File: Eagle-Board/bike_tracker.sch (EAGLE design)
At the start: 89 parts, among them IC1 24C00TS, IC2 BME280, J1 TRANSFLASH-LOCK, Q1 IRLML5203, Q2 IRLML5203, Q3 IRLML5203, Q4 IRLML5203, U1 MPU-9250

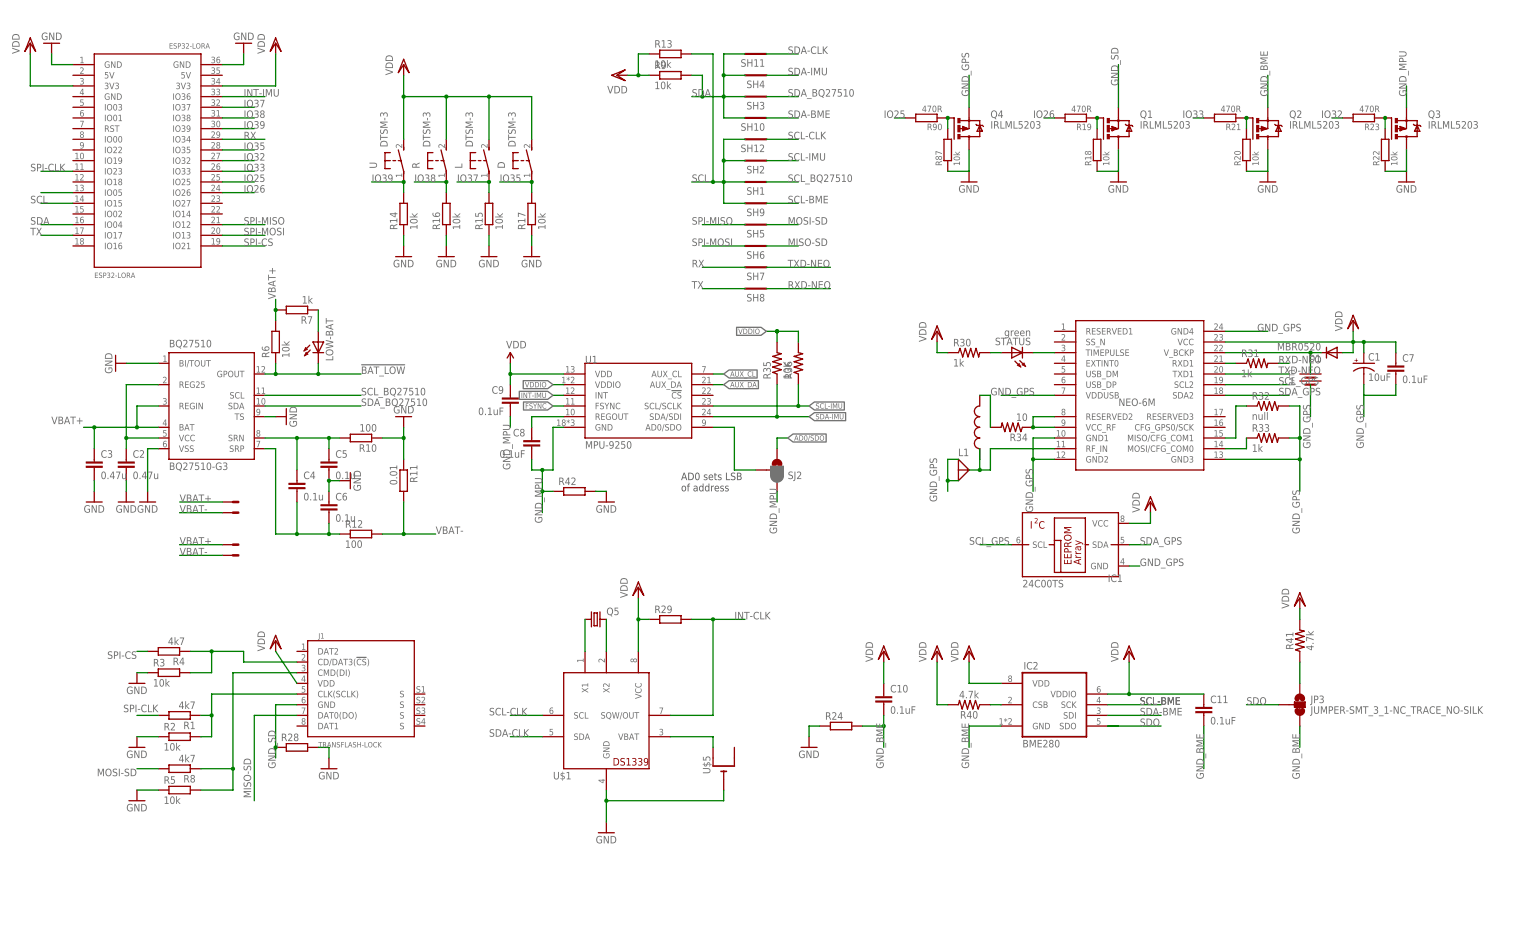
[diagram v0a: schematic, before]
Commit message: modified and cleaned for production
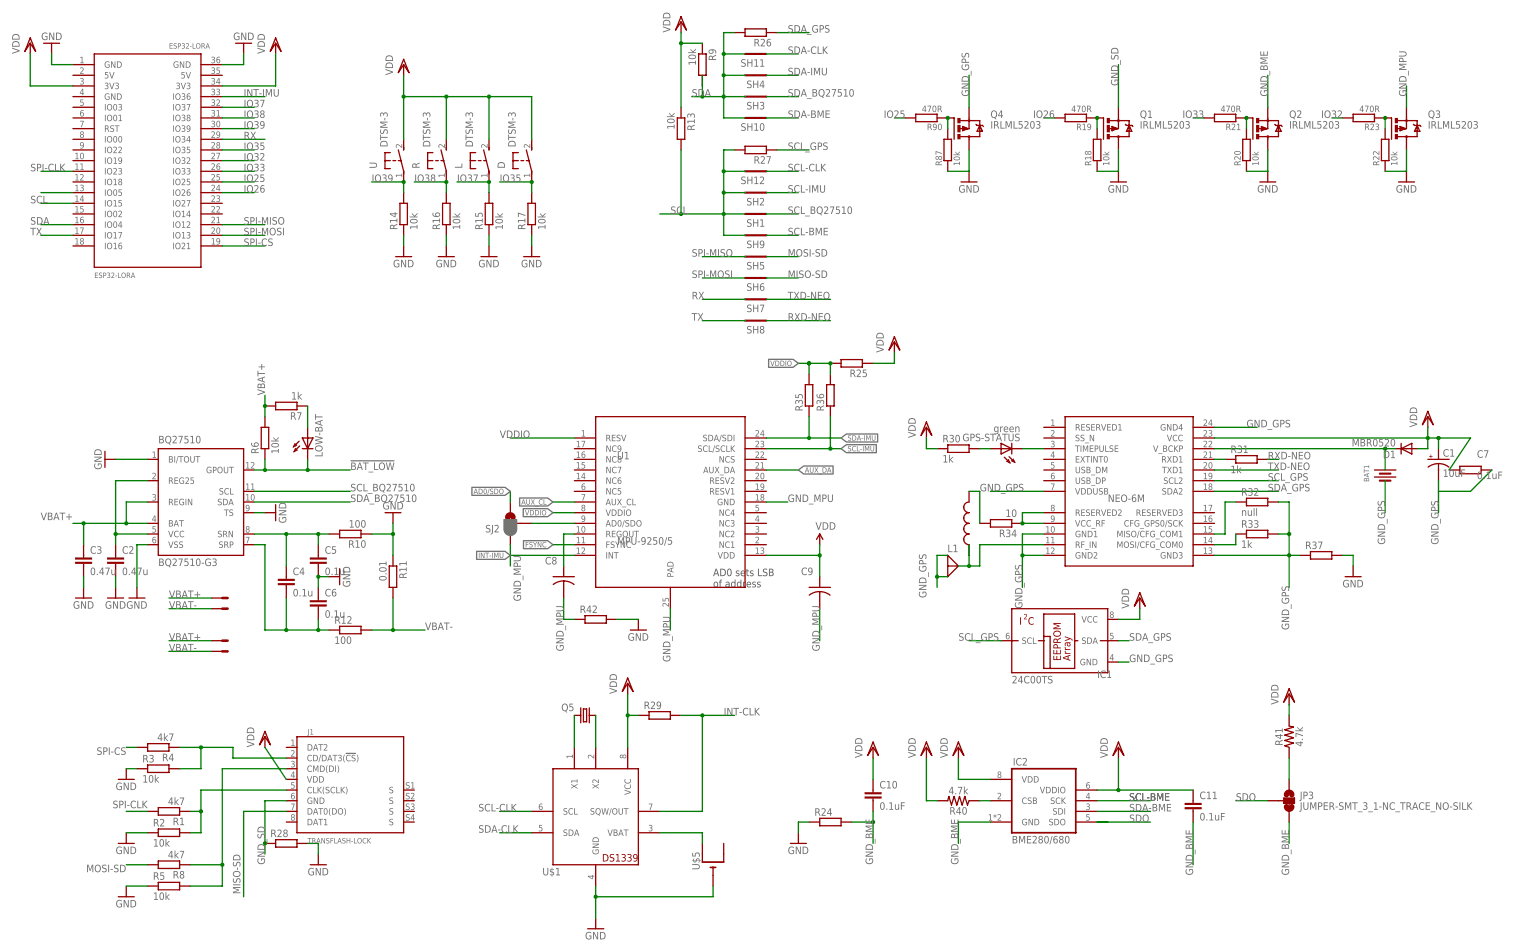
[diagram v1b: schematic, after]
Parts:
- removed STATUS: green, microduino:LED0805
- removed U$6: BLOX-NEO-6M, microduino:BLOX-NEO-6M
- added GPS-STATUS: green, microduino:LED0805
- added NEO-GPS: BLOX-NEO-6M, microduino:BLOX-NEO-6M
- added R25, R26, R27, R37: (no value), resistor:R-EU_R0201
- C7: device microduino:CAP0603-CAP -> rcl:R-EU_R0603
- C8, C9: device SparkFun-Capacitors:0.1UF-25V(+80/-20%)(0603) -> resistor:C-USC0603K
- IC2: value BME280 -> BME280/680
- R18, R19, R22, R23, R87, R90: device ssmd:R_SMDR0603 -> resistor:R-EU_R0603
- R20, R21: device ssmd:R_SMDR0603 -> rcl:R-EU_R0603
- R30: device microduino:RESISTOR0603-RES -> resistor:R-EU_R0603
- R31, R32, R33, R34: device microduino:RESISTOR0603-RES -> rcl:R-EU_R0603
- R35, R36: device SparkFun-Resistors:10KOHM-1/10W-1%(0603)0603 -> resistor:R-EU_R0603
- U1: value MPU-9250 -> MPU-9250/5; device Testing:MPU-9250 -> invensense:MPU-9250
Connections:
- net ADSD_STUB renamed N$27
- net GND: now also R37.2
- net GND_GPS: now also NEO-GPS.GND1, NEO-GPS.GND2, NEO-GPS.GND3, NEO-GPS.GND4, NEO-GPS.VDDUSB, R37.1; no longer U$6.GND1, U$6.GND2, U$6.GND3, U$6.GND4, U$6.VDDUSB
- net GND_MPU: now also U1.PAD
- net N$10: now also U$1.X2; no longer U$1.X1
- net N$13: now also U$1.X1; no longer U$1.X2
- net N$16: now also GPS-STATUS.A; no longer STATUS.A
- net N$17: now also GPS-STATUS.C, NEO-GPS.TIMEPULSE; no longer STATUS.C, U$6.TIMEPULSE
- net N$18: now also NEO-GPS.RF_IN; no longer U$6.RF_IN
- net N$19: now also NEO-GPS.RXD1; no longer U$6.RXD1
- net N$20: now also NEO-GPS.MISO/CFG_COM1; no longer U$6.MISO/CFG_COM1
- net N$21: now also NEO-GPS.MOSI/CFG_COM0; no longer U$6.MOSI/CFG_COM0
- net N$22: now also NEO-GPS.V_BCKP; no longer U$6.V_BCKP
- net N$24: now also NEO-GPS.RESERVED2, NEO-GPS.VCC_RF; no longer U$6.RESERVED2, U$6.VCC_RF
- net SCL: now also R27.2
- net SCL_GPS: now also NEO-GPS.SCL2, R27.1; no longer U$6.SCL2
- net SDA: now also R26.2
- net SDA_GPS: now also NEO-GPS.SDA2, R26.1; no longer U$6.SDA2
- net TXD-NEO: now also NEO-GPS.TXD1; no longer U$6.TXD1
- net VDD: now also NEO-GPS.VCC, R25.1; no longer U$6.VCC
- net VDDIO: now also R25.2, U1.RESV
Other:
- moved on the sheet: BAT1, BQ27510, C1, C10, C11, C2, C3, C4, C5, C6, C7, C8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
